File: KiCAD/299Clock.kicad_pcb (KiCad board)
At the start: 2 copper layers, 65 x 80 mm, 32 parts, among them SW1 PEC11R, U1 RPi Pico, U2 RDA5807M, U3 LM386

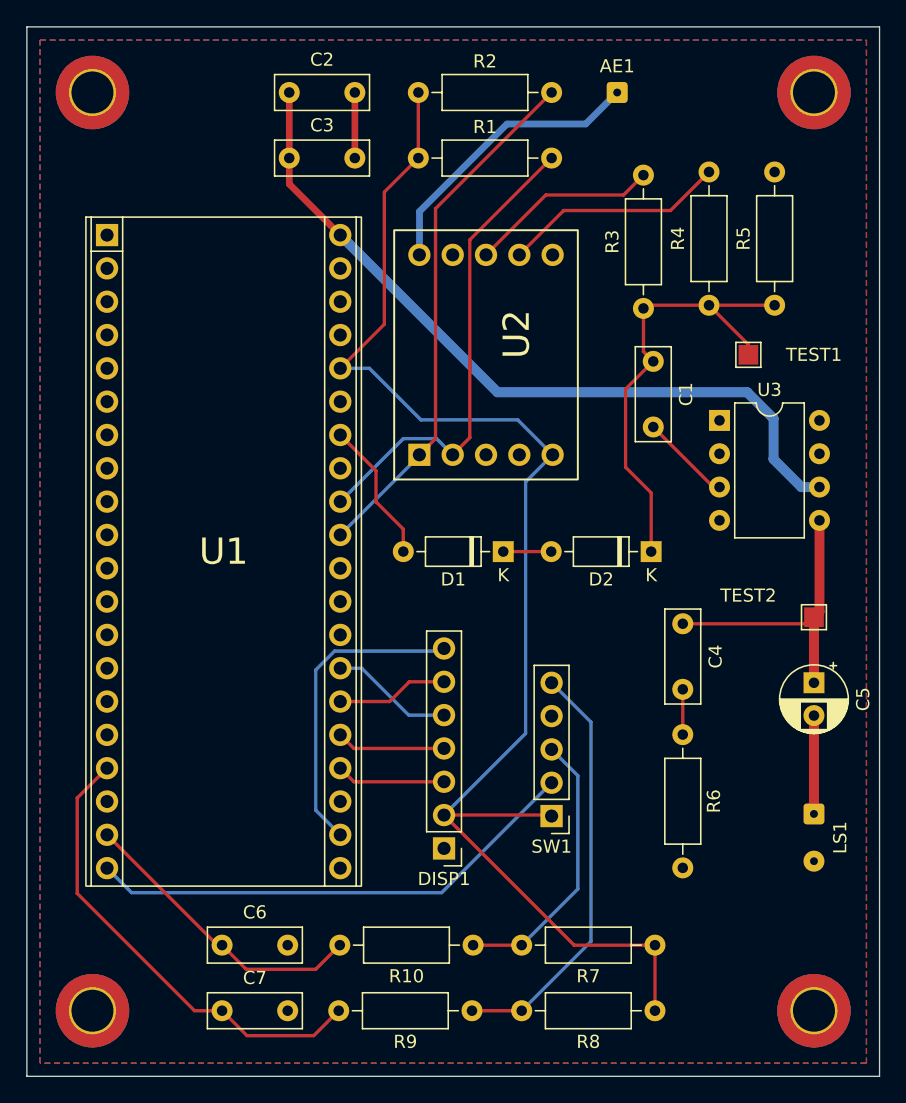
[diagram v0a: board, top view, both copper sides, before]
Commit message: revision of PCB and exported gerber
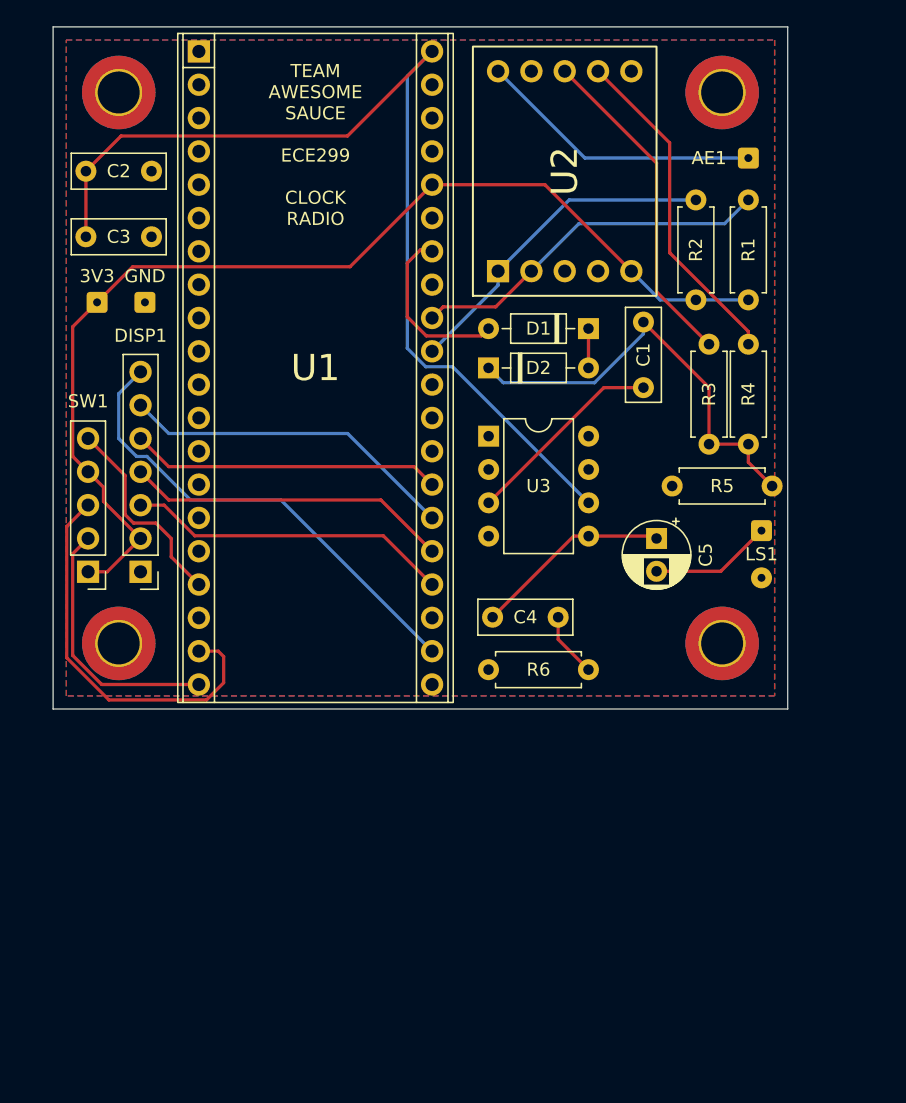
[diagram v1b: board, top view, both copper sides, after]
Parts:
- removed C6, C7: 10n, Capacitor_THT:C_Rect_L7.0mm_W2.5mm_P5.00mm
- removed R10, R7, R8, R9: 10k, Resistor_THT:R_Axial_DIN0207_L6.3mm_D2.5mm_P10.16mm_Horizontal
- removed TEST1, TEST2: Conn_01x01, TestPoint:TestPoint_Pad_1.5x1.5mm
- added 3V3: 3V3, Connector_Wire:SolderWire-0.1sqmm_1x01_D0.4mm_OD1mm, F.Cu at (100.3, 71.0)
- added GND: GND, Connector_Wire:SolderWire-0.1sqmm_1x01_D0.4mm_OD1mm, F.Cu at (104.0, 71.0)
- R1, R2, R3, R4, R5, R6: footprint Resistor_THT:R_Axial_DIN0207_L6.3mm_D2.5mm_P10.16mm_Horizontal -> Resistor_THT:R_Axial_DIN0207_L6.3mm_D2.5mm_P7.62mm_Horizontal
- moved SW1 39.9 mm to (99.7, 91.5)
- moved DISP1 31.3 mm to (103.7, 91.5)
- moved H4 28.9 mm to (148.0, 97.0)
- moved H3 28.1 mm to (102.0, 97.0)
- moved R1 27.4 mm to (150.0, 70.8), turned to 90 degrees
- moved R2 26.4 mm to (146.0, 70.8), turned to 90 degrees
- moved LS1 22.0 mm to (151.0, 88.4)
- moved D2 18.7 mm to (130.2, 76.0), turned to 0 degrees
- moved D1 18.2 mm to (137.8, 73.0)
- moved U3 17.6 mm to (130.2, 81.2)
- moved C2 16.6 mm to (99.5, 61.0)
- moved C3 16.6 mm to (99.5, 66.0)
- moved C5 16.3 mm to (143.0, 89.0)
- moved U1 15.7 mm to (117.0, 76.0)
- moved U2 15.2 mm to (136.0, 61.0)
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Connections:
- SW1 pad A: Net-(R10-Pad1) -> Net-(SW1-PadA)
- SW1 pad B: Net-(R8-Pad2) -> Net-(SW1-PadB)
- SW1 pad C: GND -> Net-(DISP1-Pad2)
- U1 pad 17: Net-(C7-Pad1) -> Net-(SW1-PadB)
- U1 pad 19: Net-(C6-Pad1) -> Net-(SW1-PadA)
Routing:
- net Net-(C7-Pad1): track 35.7 -> 0.00 mm
- net Net-(R8-Pad2): track 32.2 -> 0.00 mm
- net Net-(SW1-PadA): track 0.00 -> 30.2 mm
- net Net-(DISP1-Pad2): track 106.7 -> 83.0 mm
- net Net-(C6-Pad1): track 22.8 -> 0.00 mm
- net Net-(R10-Pad1): track 21.2 -> 0.00 mm
- net Net-(C2-Pad1): track 58.8 -> 77.3 mm
- net Net-(SW1-PadS2): track 38.1 -> 19.9 mm
- net Net-(DISP1-Pad6): track 8.53 -> 25.8 mm
- net Net-(DISP1-Pad4): track 8.34 -> 24.7 mm
- net Net-(DISP1-Pad3): track 8.34 -> 24.7 mm
- net Net-(SW1-PadB): track 0.00 -> 15.6 mm
- net Net-(R2-Pad2): track 40.4 -> 25.5 mm
- net Net-(DISP1-Pad5): track 9.39 -> 23.7 mm
- net Net-(DISP1-Pad7): track 23.8 -> 36.4 mm
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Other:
- board size 65 x 80 mm -> 56 x 52 mm
- board text added: "TEAM AWESOME SAUCE ECE299 CLOCK RADIO"
